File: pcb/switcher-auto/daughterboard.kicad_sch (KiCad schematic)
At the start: 6 parts, among them J0 MD-90SM, J1 MD-90SM, J2 MD-90SM, J3 MD-90SM, J4 MD-90SM, J5 Conn_02x22_Top_Bottom

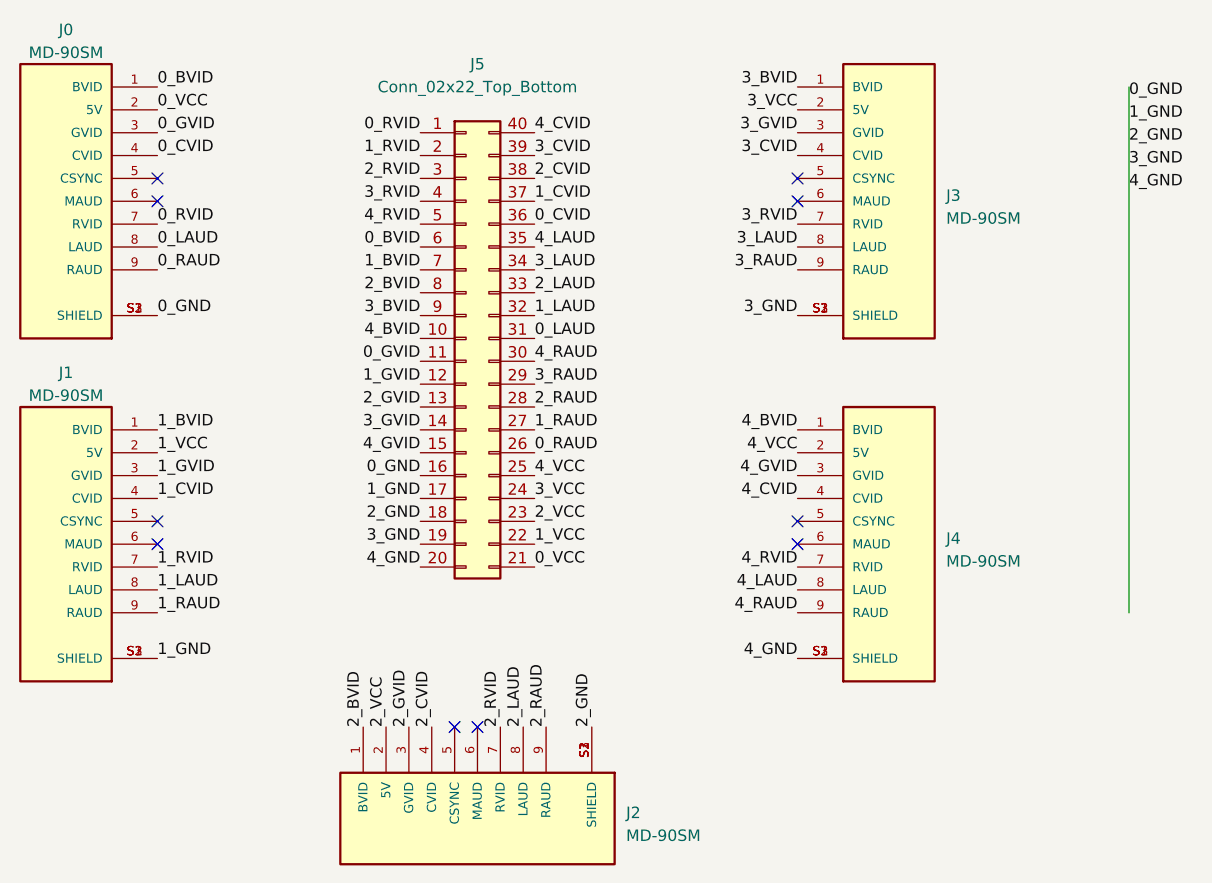
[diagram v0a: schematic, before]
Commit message: Routing pt 2
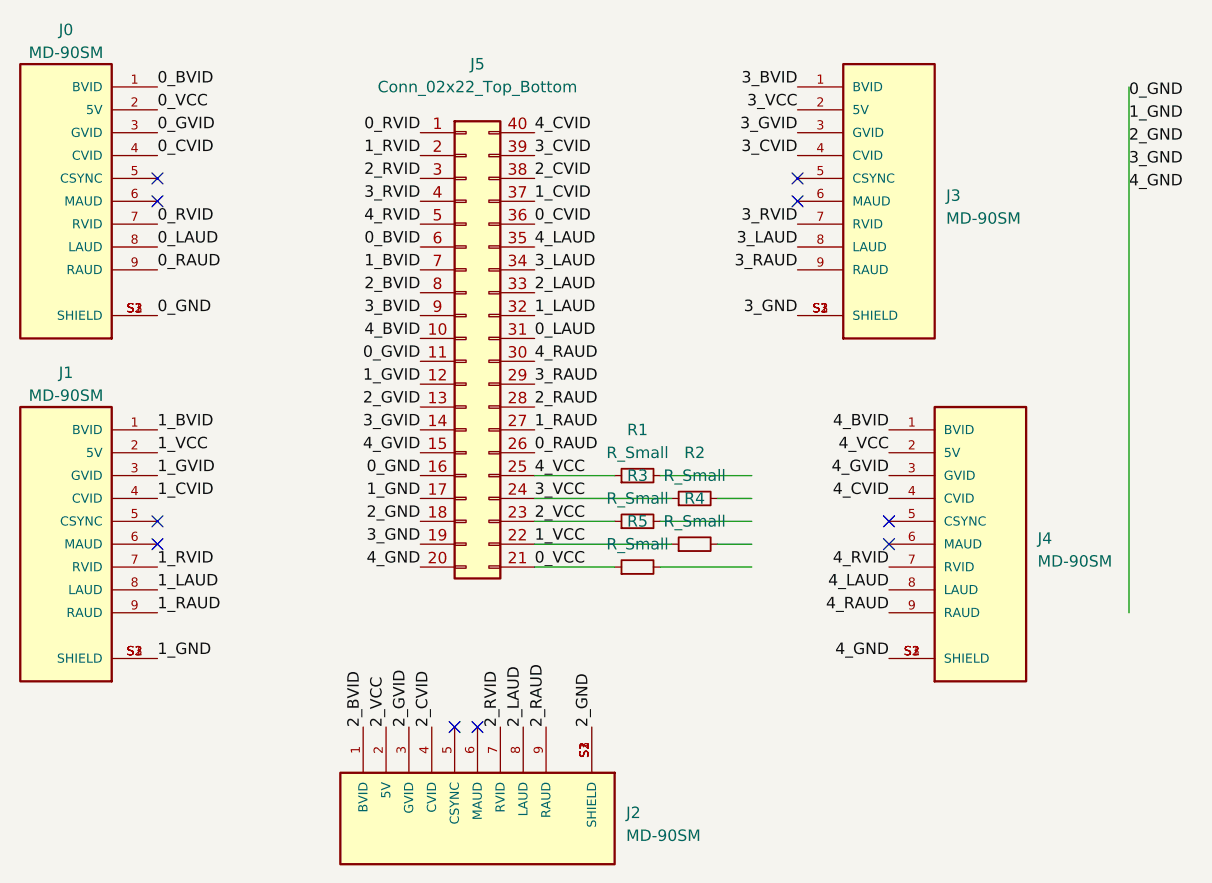
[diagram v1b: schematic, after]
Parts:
- added R1, R2, R3, R4, R5: R_Small, Resistor_SMD:R_0805_2012Metric_Pad1.20x1.40mm_HandSolder, symbol Device:R_Small
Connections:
- net 0_VCC: now also R5.1
- net 1_VCC: now also R4.1
- net 2_VCC: now also R3.1
- net 3_VCC: now also R2.1
- net 4_VCC: now also R1.1
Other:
- moved on the sheet: J4
